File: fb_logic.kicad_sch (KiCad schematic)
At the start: 10 parts, among them U1 74LS14, U2 74LS74, U3 74LS08, U4 LM311, U5 TL3116

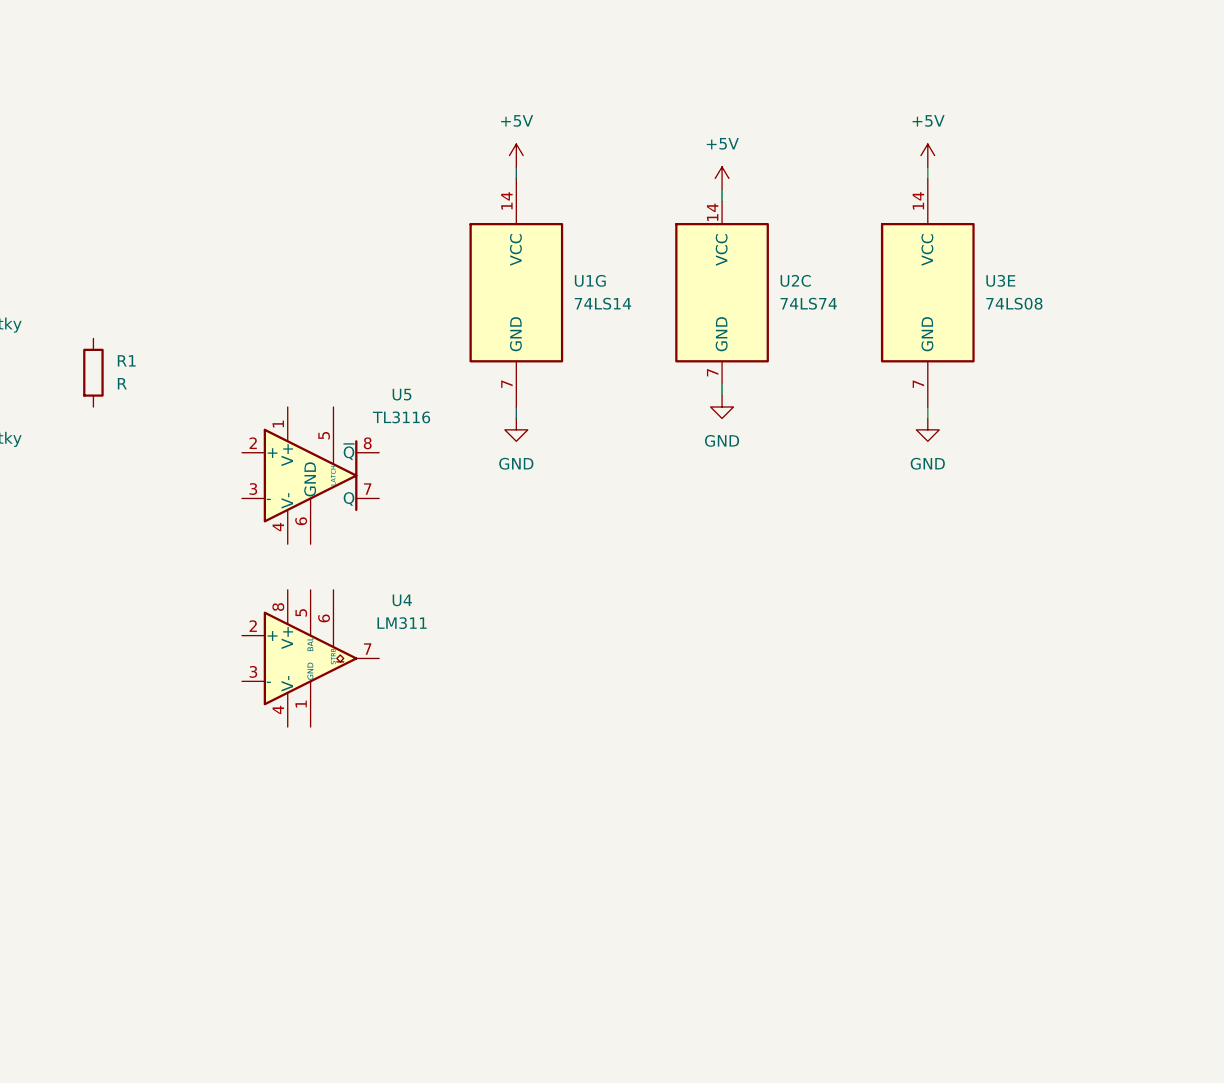
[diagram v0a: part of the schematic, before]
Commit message: added progress
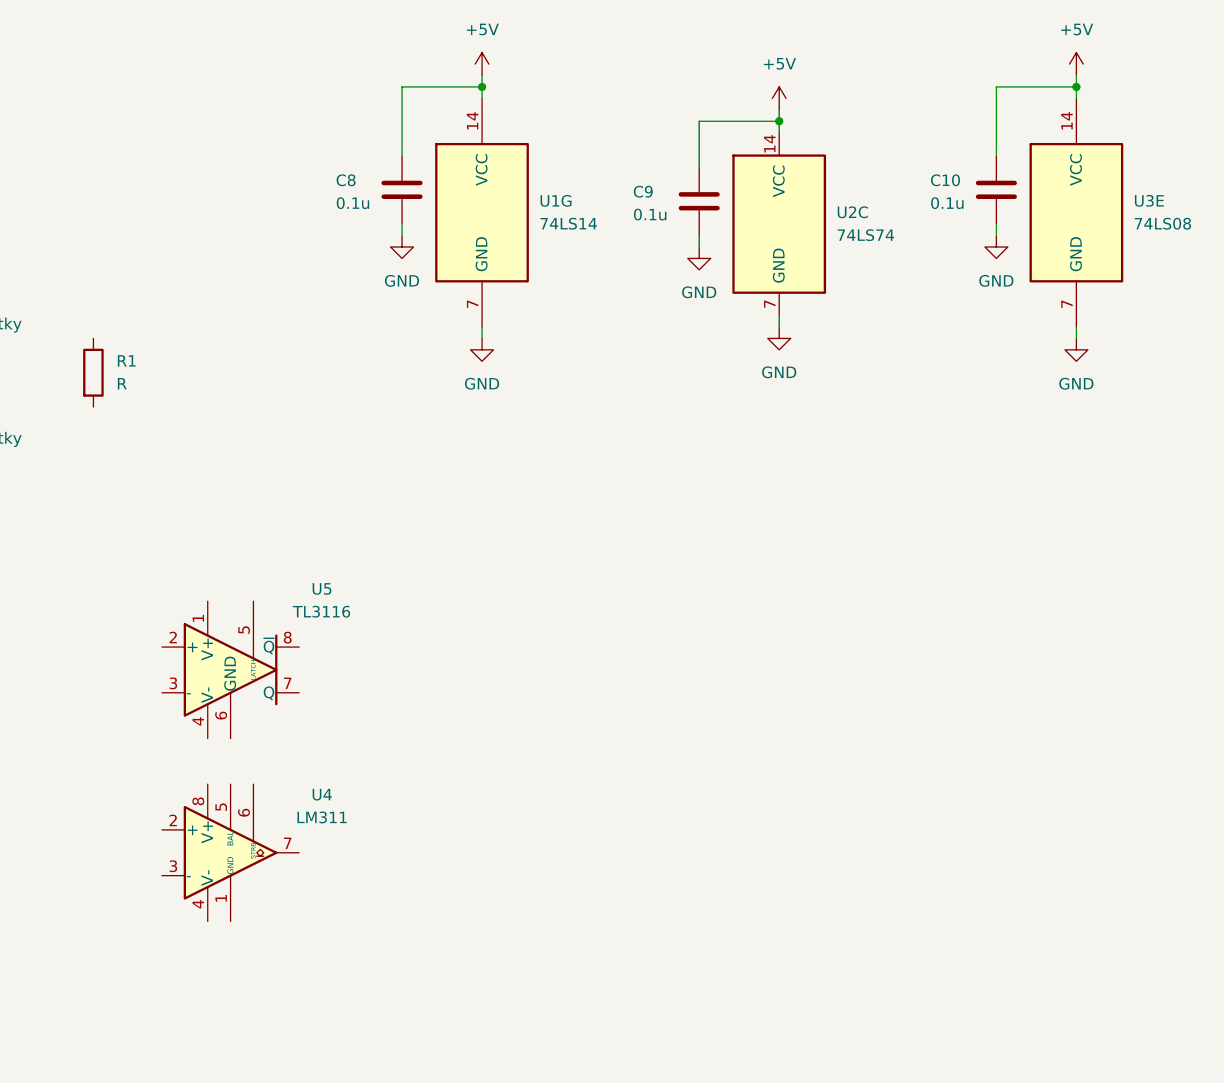
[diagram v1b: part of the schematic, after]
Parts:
- added C10, C8, C9: 0.1u, symbol Device:C
- R1: footprint (none) -> Resistor_SMD:R_0805_2012Metric
- U4: footprint (none) -> Package_DIP:DIP-8_W7.62mm_Socket
- U5: footprint (none) -> Package_SO:SOIC-8_3.9x4.9mm_P1.27mm
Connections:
- net +5V: now also C10.2, C8.2, C9.2
- net GND: now also C10.1, C8.1, C9.1
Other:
- moved on the sheet: U1G, U2C, U3E, U4, U5

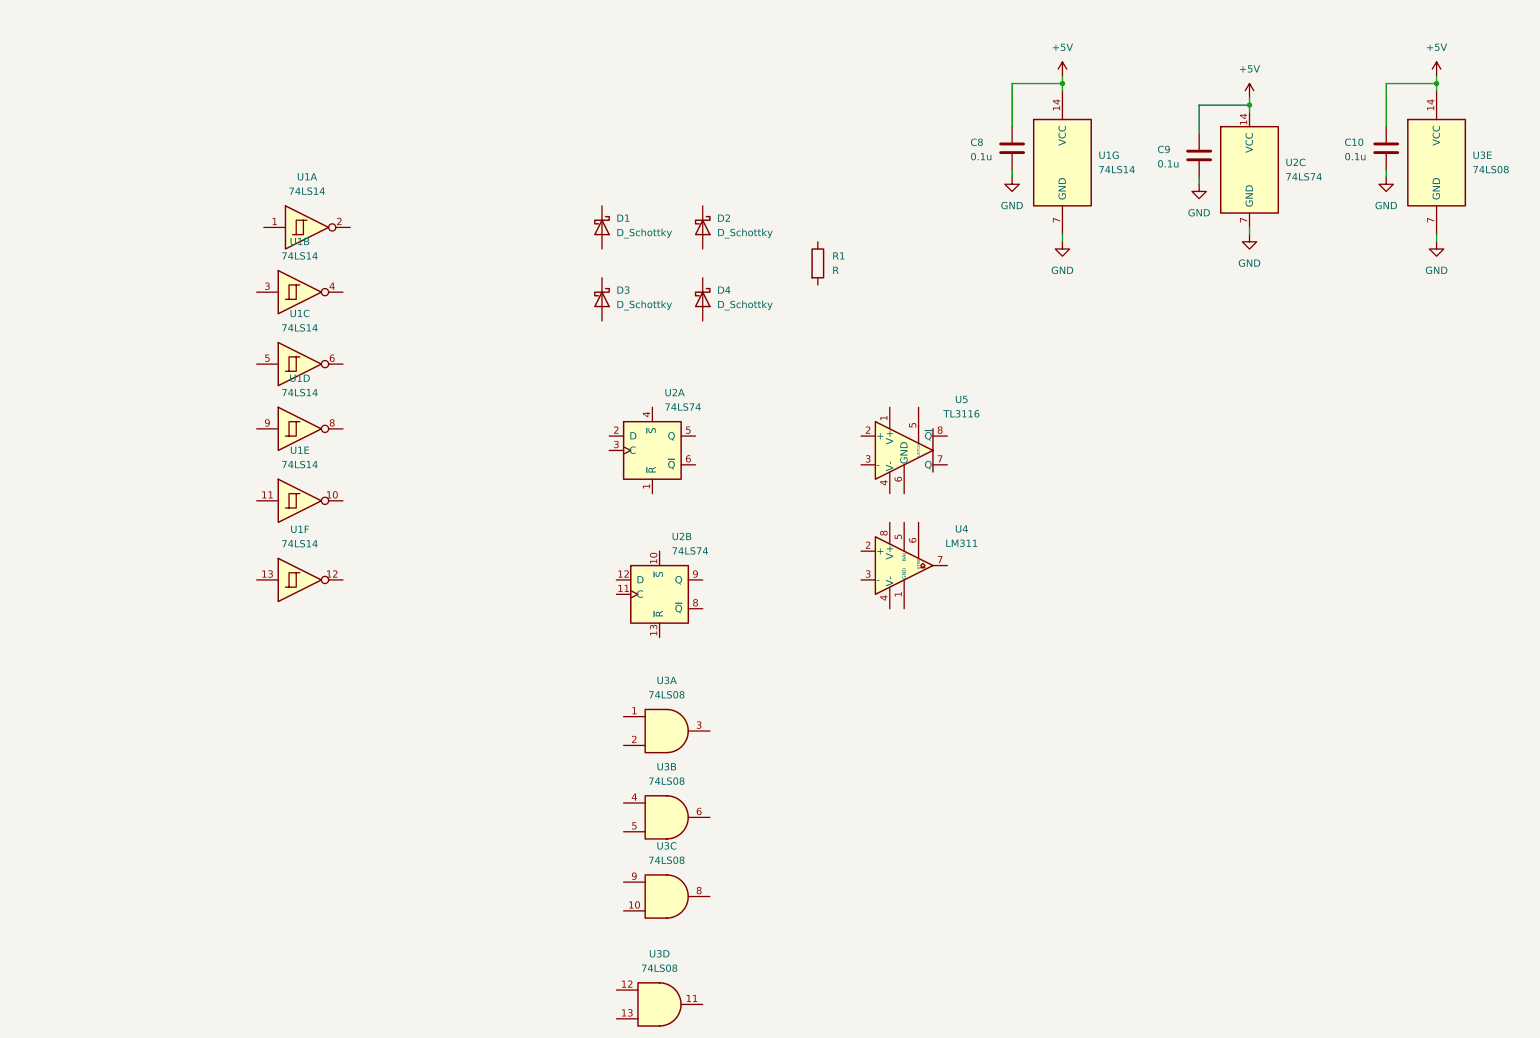
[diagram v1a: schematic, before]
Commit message: large amount of work
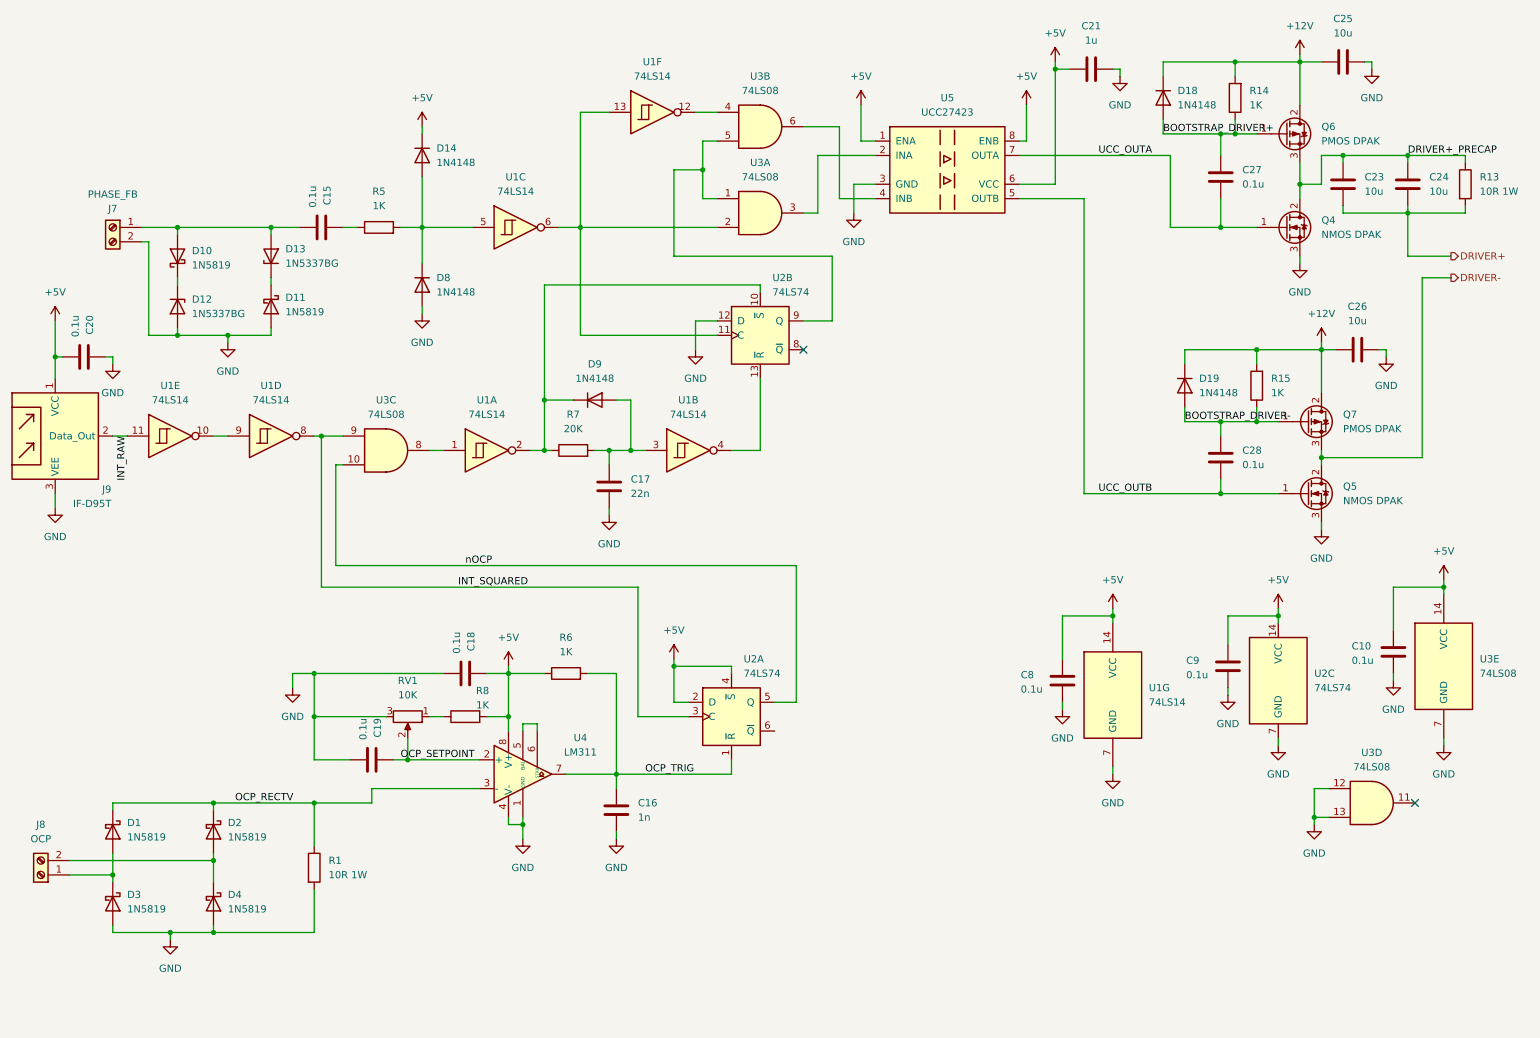
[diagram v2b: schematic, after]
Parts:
- removed U5: TL3116, Package_SO:SOIC-8_3.9x4.9mm_P1.27mm, symbol Comparator:TL3116
- added C15, C18, C19, C20, C27, C28: 0.1u, Capacitor_SMD:C_0805_2012Metric, symbol Device:C
- added C16: 1n, Capacitor_SMD:C_0805_2012Metric, symbol Device:C
- added C17: 22n, Capacitor_SMD:C_0805_2012Metric, symbol Device:C
- added C21: 1u, Capacitor_SMD:C_0805_2012Metric, symbol Device:C
- added C23, C24, C25, C26: 10u, Capacitor_SMD:C_1206_3216Metric, symbol Device:C
- added D10, D11: 1N5819, Diode_THT:D_DO-41_SOD81_P2.54mm_Vertical_AnodeUp, symbol Device:D_Schottky
- added D12, D13: 1N5337BG, Diode_THT:D_5KPW_P7.62mm_Vertical_AnodeUp, symbol Device:D_Zener
- added D14, D18, D19, D8, D9: 1N4148, Diode_THT:D_DO-35_SOD27_P2.54mm_Vertical_AnodeUp, symbol Diode:1N4148
- added J7: PHASE_FB, TerminalBlock_Phoenix:TerminalBlock_Phoenix_MKDS-1,5-2_1x02_P5.00mm_Horizontal, symbol Connector:Screw_Terminal_01x02
- added J8: OCP, TerminalBlock_Phoenix:TerminalBlock_Phoenix_MKDS-1,5-2_1x02_P5.00mm_Horizontal, symbol Connector:Screw_Terminal_01x02
- added J9: IF-D95T, Package_TO_SOT_THT:TO-92_Inline_Wide, symbol Fiber_Optic:AFBR-2624Z
- added Q4, Q5: NMOS DPAK, Package_TO_SOT_SMD:TO-252-2, symbol Transistor_FET:STD7NK40Z
- added Q6, Q7: PMOS DPAK, Package_TO_SOT_SMD:TO-252-2, symbol Transistor_FET:QM6015D
- added R13: 10R 1W, Resistor_SMD:R_2512_6332Metric, symbol Device:R
- added R14, R15, R5, R6, R8: 1K, Resistor_SMD:R_0805_2012Metric, symbol Device:R
- added R7: 20K, Resistor_SMD:R_0805_2012Metric, symbol Device:R
- added RV1: 10K, Potentiometer_THT:Potentiometer_Bourns_3386P_Vertical, symbol Device:R_Potentiometer
- added U5: UCC27423, Package_SO:SOIC-8_3.9x4.9mm_P1.27mm, symbol Isolator:ADuM120N
- C10, C8, C9: footprint (none) -> Capacitor_SMD:C_0805_2012Metric
- D1, D2, D3, D4: value D_Schottky -> 1N5819; footprint (none) -> Diode_THT:D_DO-41_SOD81_P2.54mm_Vertical_AnodeUp
- R1: value R -> 10R 1W; footprint Resistor_SMD:R_0805_2012Metric -> Resistor_SMD:R_2512_6332Metric
- U1, U2, U3: footprint Package_DIP:DIP-14_W7.62mm_Socket -> Package_SO:SOIC-14_3.9x8.7mm_P1.27mm
- U4: footprint Package_DIP:DIP-8_W7.62mm_Socket -> Package_SO:SOIC-8_3.9x4.9mm_P1.27mm
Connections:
- net +5V: now also U2.2 (D), U2.4 (~{S}), U4.8 (V+), C18.2, C20.1, C21.1, D14.1 (K), J9.1 (VCC), R6.1, R8.2, U5.1 (ENA), U5.6 (VCC), U5.8 (ENB)
- net GND: now also D3.2 (A), D4.2 (A), R1.2, U2.12 (D), U3.12, U3.13, U4.1 (GND), U4.4 (V-), C16.2, C17.2, C18.1, C19.1, C20.2, C21.2, C25.2, C26.2, D11.2 (A), D12.2 (A), D8.2 (A), J7.2 (Pin_2), J9.3 (VEE), Q4.3 (S), Q5.3 (S), RV1.3, U5.3 (GND)
- net at U1.12: now also U3.4
- net at U1.13: now also U1.6, U2.11 (C), U3.2
- net OCP_SETPOINT: now reaches U4.2 (+)
- net OCP_SETPOINT: now also C19.2, RV1.2
- net OCP_RECTV: now reaches U4.3 (-)
- net OCP_RECTV: now also D1.1 (K), D2.1 (K), R1.1
- net at U4.5 (BAL): now also U4.6 (STRB)
- net OCP_TRIG: now reaches U4.7
- net OCP_TRIG: now also U2.1 (~{R}), C16.1, R6.2
- net INT_SQUARED: now reaches U1.8
- net INT_SQUARED: now also U2.3 (C), U3.9
- net at U1.9: now also U1.10
- net at D1.2 (A): now also D3.1 (K), J8.1 (Pin_1)
- net at D2.2 (A): now also D4.1 (K), J8.2 (Pin_2)
- net at U1.5: now also D14.2 (A), D8.1 (K), R5.2
- net at U3.5: now also U2.9 (Q), U3.1
- net at U3.6: now also U5.4 (INB)
- net nOCP: now reaches U2.5 (Q)
- net nOCP: now also U3.10
- net at U3.8: now also U1.1
- net at U1.3: now also C17.1, D9.2 (A), R7.2
- net at U1.4: now also U2.13 (~{R})
- net at U3.3: now also U5.2 (INA)
- net at U1.2: now also U2.10 (~{S}), D9.1 (K), R7.1
- net INT_RAW: now reaches U1.11
- net INT_RAW: now also J9.2 (Data_Out)
- new net: D10.1 (K), D12.1 (K)
- new net: C15.1, D10.2 (A), D13.2 (A), J7.1 (Pin_1)
- new net: C15.2, R5.1
- new net: D11.1 (K), D13.1 (K)
- new net: R8.1, RV1.1
- new net +12V: C25.1, C26.1, D18.1 (K), D19.1 (K), Q6.2 (D), Q7.2 (D), R14.2, R15.2
- new net BOOTSTRAP_DRIVER+: C27.2, D18.2 (A), Q6.1 (G), R14.1
- new net BOOTSTRAP_DRIVER-: C28.2, D19.2 (A), Q7.1 (G), R15.1
- new net DRIVER+: C23.2, C24.2, R13.2
- new net DRIVER+_PRECAP: C23.1, C24.1, Q4.2 (D), Q6.3 (S), R13.1
- new net DRIVER-: Q5.2 (D), Q7.3 (S)
- new net UCC_OUTA: C27.1, Q4.1 (G), U5.7 (OUTA)
- new net UCC_OUTB: C28.1, Q5.1 (G), U5.5 (OUTB)
- no-connect marks 0 -> 2
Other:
- moved on the sheet: C10, C8, C9, D1, D2, D3, D4, R1, U1B, U1G, U2C, U3E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
